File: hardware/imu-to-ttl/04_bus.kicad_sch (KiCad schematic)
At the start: 9 parts, among them U3 SN74LVC1G125DBVT

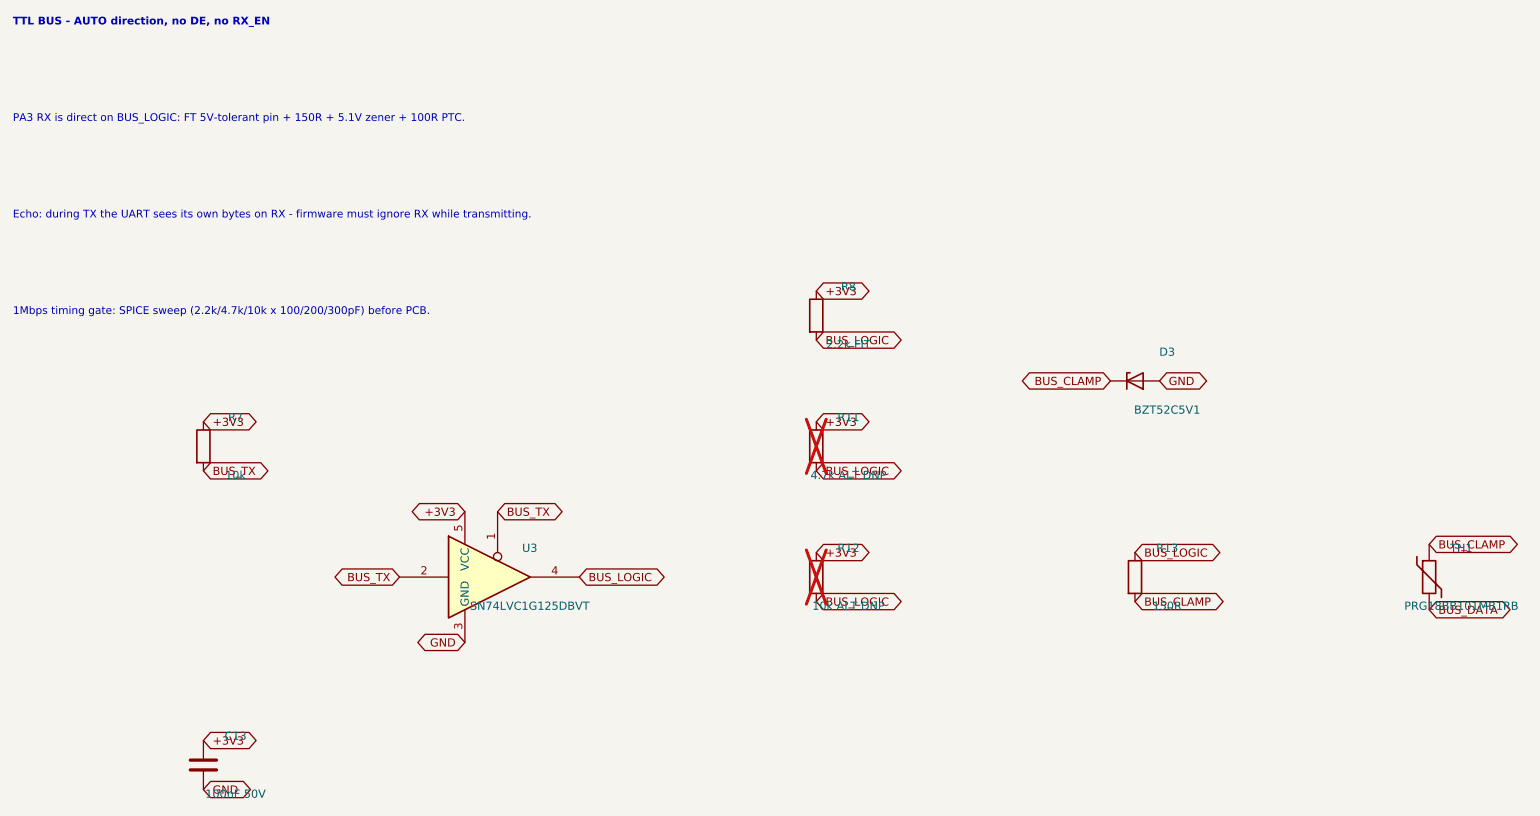
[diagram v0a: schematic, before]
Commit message: sync: 2026-10-15 日常更新
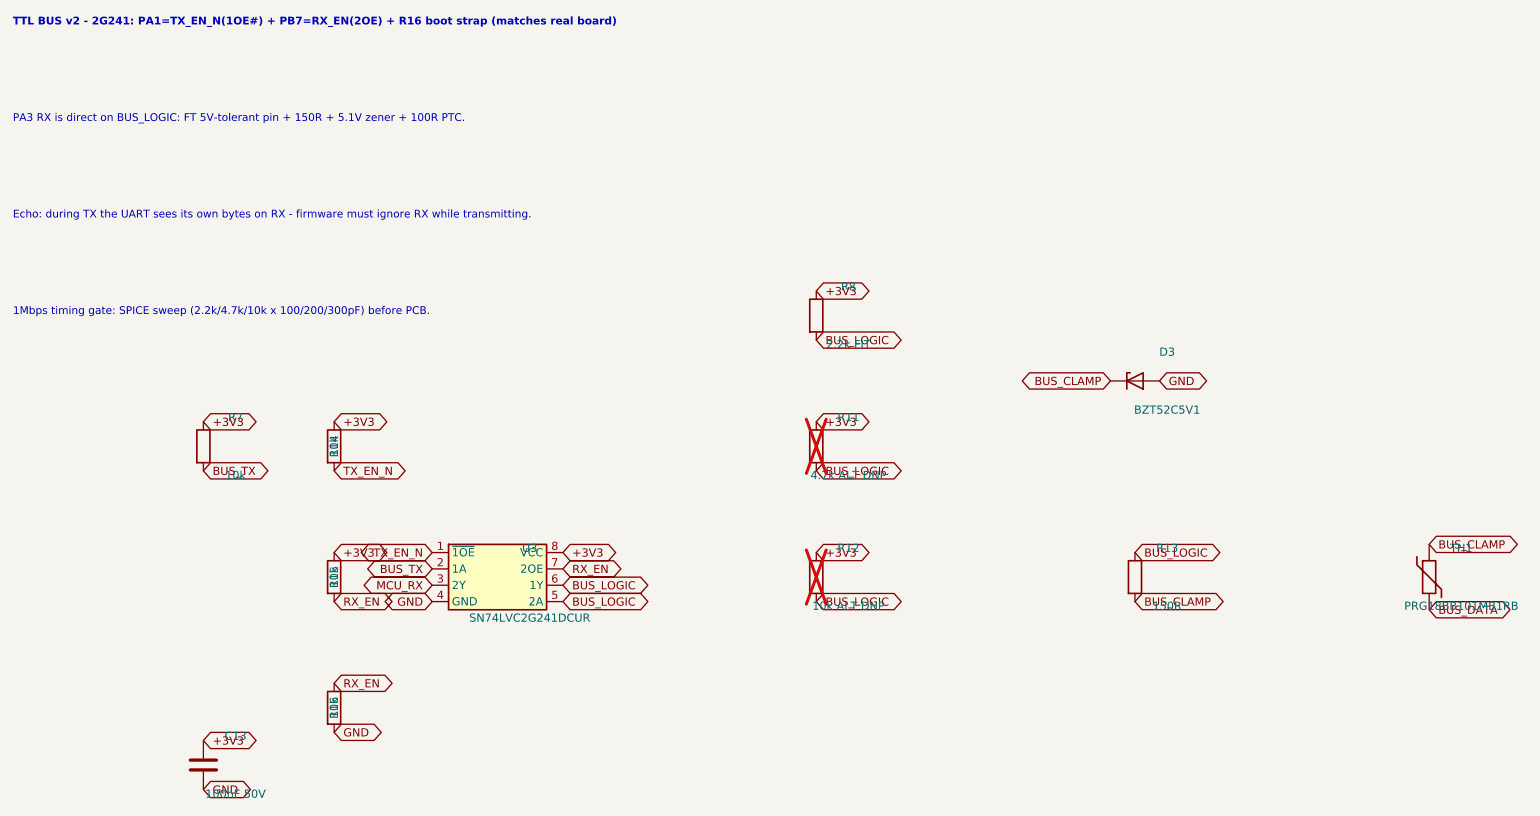
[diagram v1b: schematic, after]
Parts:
- removed U3: SN74LVC1G125DBVT, Package_TO_SOT_SMD:SOT-23-5, symbol 74xGxx:74LVC1G125
- added R14, R15, R16: 10k, Resistor_SMD:R_0603_1608Metric, symbol Device:R
- added U3: SN74LVC2G241DCUR, Package_SO:TSSOP-8_3x3mm_P0.65mm, symbol 74xGxx:SN74LVC2G241
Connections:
- net +3V3: now also R14.1, R15.1, U3.8 (VCC)
- net BUS_LOGIC: now also U3.5 (2A), U3.6 (1Y)
- net BUS_TX: now also U3.2 (1A)
- net GND: now also R16.2, U3.4 (GND)
- new net MCU_RX: U3.3 (2Y)
- new net RX_EN: R15.2, R16.1, U3.7 (2OE)
- new net TX_EN_N: R14.2, U3.1 (~{1OE})
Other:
- note added: "TTL BUS v2 - 2G241: PA1=TX_EN_N(1OE#) + PB7=RX_EN(2OE) + R16 boot strap (matches real board)"
- note removed: "TTL BUS - AUTO direction, no DE, no RX_EN"

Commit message: sync: 2026-10-15 日常更新
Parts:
- R14, R15, R16: LCSC (none) -> C25804; MPN (none) -> 0603WAF1002T5E
- U3: footprint Package_SO:TSSOP-8_3x3mm_P0.65mm -> Package_SO:VSSOP-8_2.3x2mm_P0.5mm; LCSC (none) -> C10430
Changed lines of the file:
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@@
 		)
 	)
-	)
-		(property "Footprint" "Package_SO:TSSOP-8_3x3mm_P0.65mm"
+	)		(property "LCSC" "C10430"
+			(at 100.33 110.49 0)
+			(effects
+				(font
+					(size 1.27 1.27)
+				)
+				(hide yes)
+			)
+		)
+		(property "Footprint" "Package_SO:VSSOP-8_2.3x2mm_P0.5mm"
 		(at 100.33 110.49 0)
 		(effects
@@
 		)
 	)
-	)
+	)		(property "MPN" "0603WAF1002T5E"
+			(at 74.93 130.81 0)
+			(effects
+				(font
+					(size 1.27 1.27)
+				)
+				(hide yes)
+			)
+		)
+		(property "LCSC" "C25804"
+			(at 74.93 130.81 0)
+			(effects
+				(font
+					(size 1.27 1.27)
+				)
+				(hide yes)
+			)
+		)
 		(property "Footprint" "Resistor_SMD:R_0603_1608Metric"
 		(at 74.93 90.17 0)
@@
 		)
 	)
-	)
+	)		(property "MPN" "0603WAF1002T5E"
+			(at 74.93 130.81 0)
+			(effects
+				(font
+					(size 1.27 1.27)
+				)
+				(hide yes)
+			)
+		)
+		(property "LCSC" "C25804"
+			(at 74.93 130.81 0)
+			(effects
+				(font
+					(size 1.27 1.27)
+				)
+				(hide yes)
+			)
+		)
 		(property "Footprint" "Resistor_SMD:R_0603_1608Metric"
 		(at 74.93 110.49 0)
@@
 		)
 	)
-	)
+	)		(property "MPN" "0603WAF1002T5E"
+			(at 74.93 130.81 0)
+			(effects
+				(font
+					(size 1.27 1.27)
+				)
+				(hide yes)
+			)
+		)
+		(property "LCSC" "C25804"
+			(at 74.93 130.81 0)
+			(effects
+				(font
+					(size 1.27 1.27)
+				)
+				(hide yes)
+			)
+		)
 		(property "Footprint" "Resistor_SMD:R_0603_1608Metric"
 		(at 74.93 130.81 0)
